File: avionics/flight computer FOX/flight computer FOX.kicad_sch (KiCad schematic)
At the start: 7 parts, among them U1 ESP32-S3-DevKitC

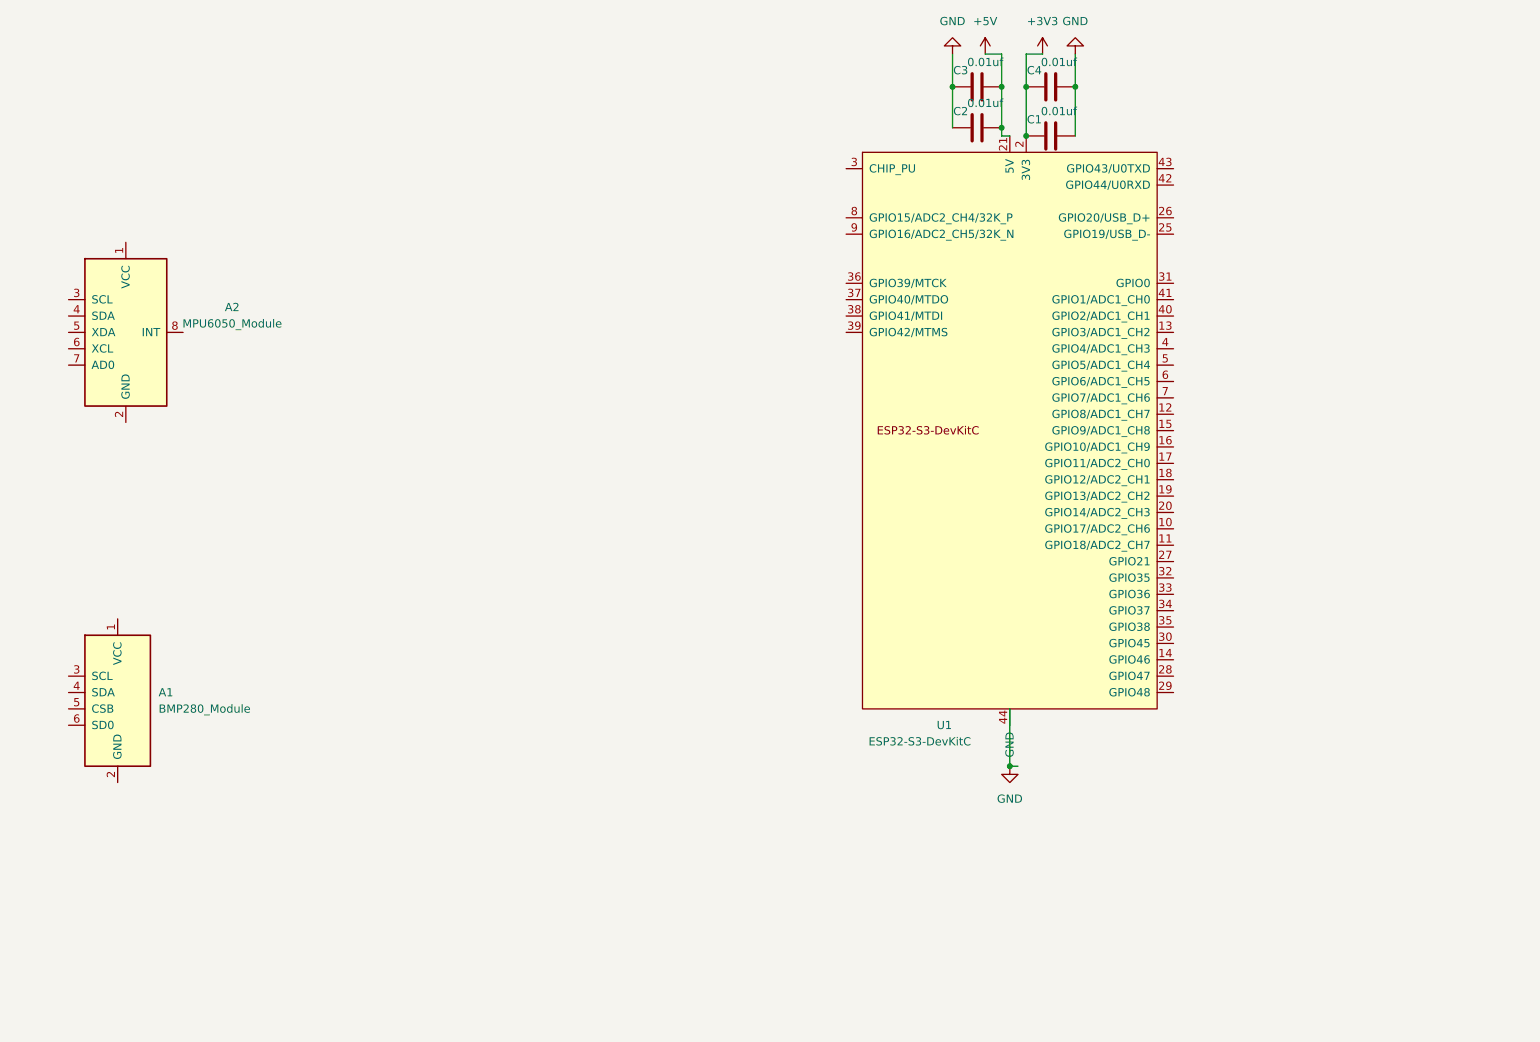
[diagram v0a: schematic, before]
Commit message: some stuff
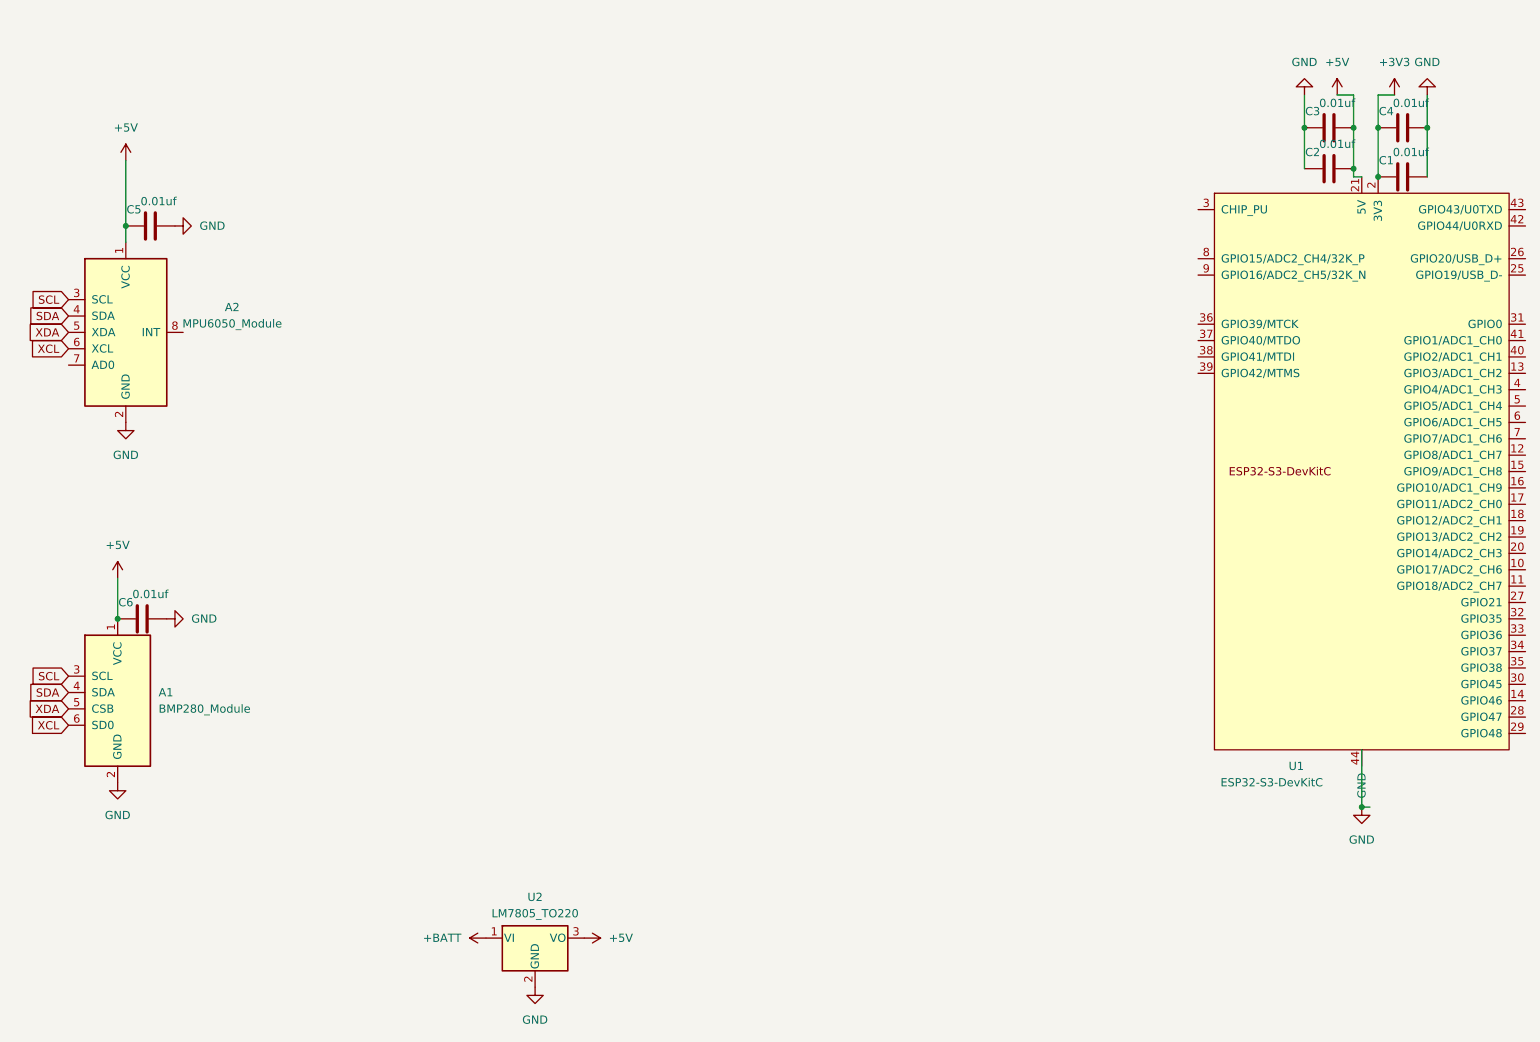
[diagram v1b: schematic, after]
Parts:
- added C5, C6: 0.01uf, symbol Device:C
- added U2: LM7805_TO220, Package_TO_SOT_THT:TO-220-3_Vertical, symbol Regulator_Linear:LM7805_TO220
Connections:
- net +5V: now also A1.1 (VCC), A2.1 (VCC), C5.1, C6.1, U2.3 (VO)
- net GND: now also A1.2 (GND), A2.2 (GND), C5.2, C6.2, U2.2 (GND)
- net SCL: now reaches A2.3 (SCL)
- net SCL: now also A1.3 (SCL)
- net SDA: now reaches A2.4 (SDA)
- net SDA: now also A1.4 (SDA)
- net XDA: now reaches A2.5 (XDA)
- net XDA: now also A1.5 (CSB)
- net XCL: now reaches A2.6 (XCL)
- net XCL: now also A1.6 (SD0)
- new net +BATT: U2.1 (VI)
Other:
- moved on the sheet: C1, C2, C3, C4, U1

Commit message: more flight computer work
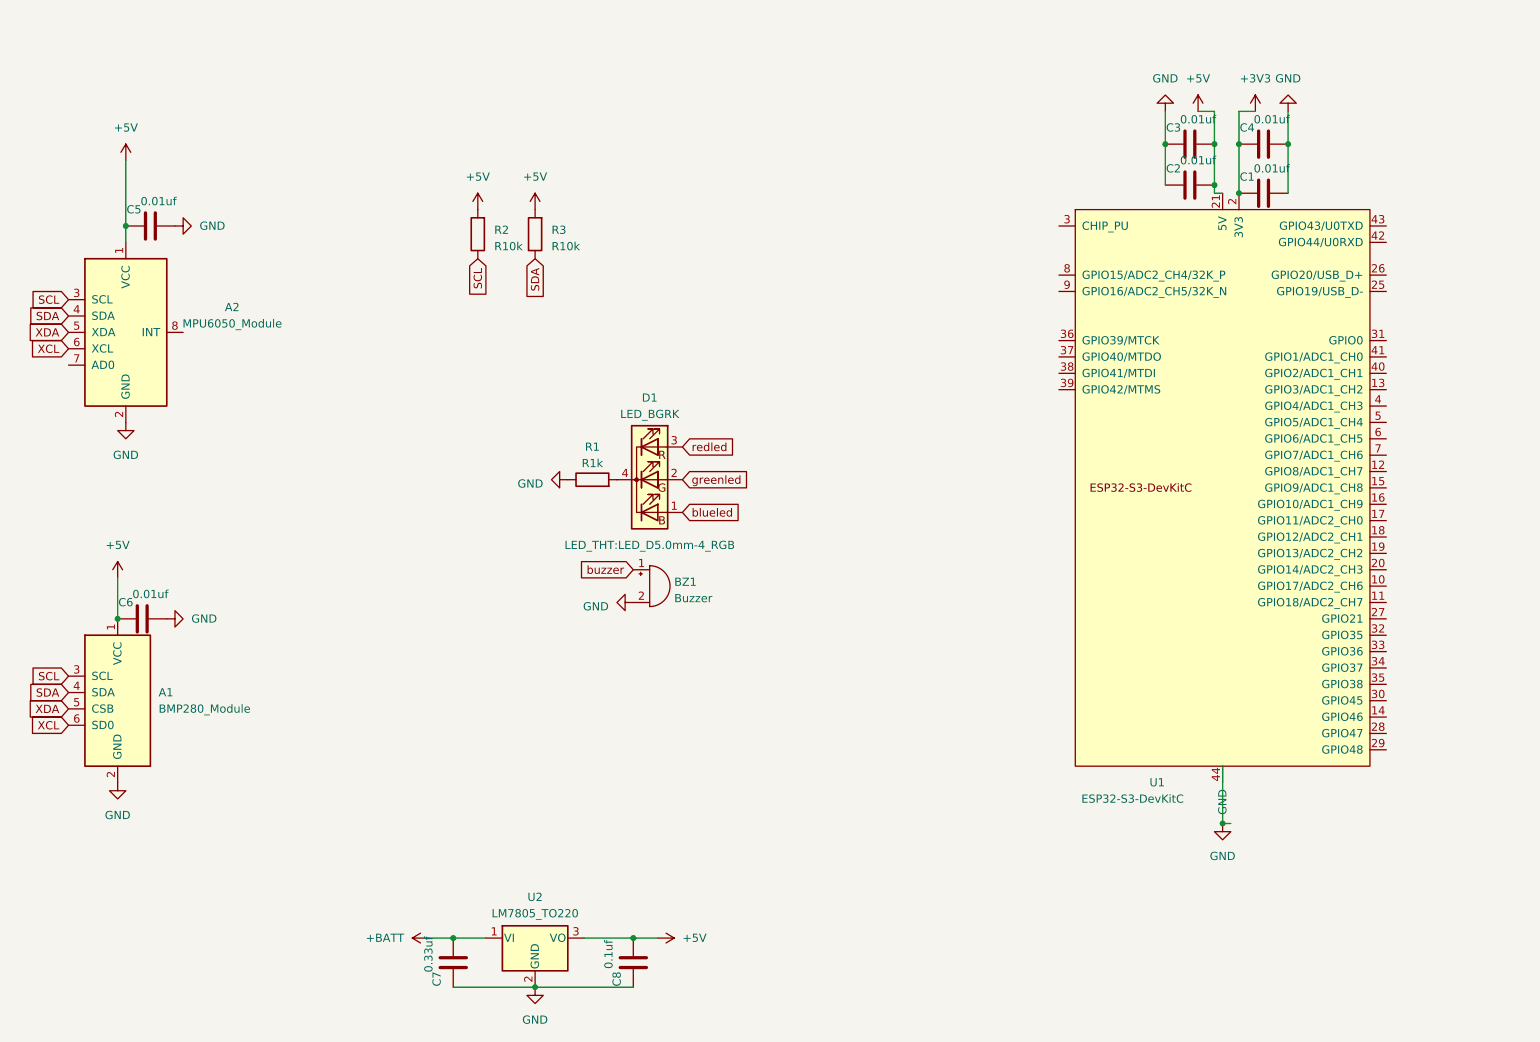
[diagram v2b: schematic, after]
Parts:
- added BZ1: Buzzer, Buzzer_Beeper:Buzzer_12x9.5RM7.6, symbol Device:Buzzer
- added C7: 0.33uf, Capacitor_SMD:C_0805_2012Metric_Pad1.18x1.45mm_HandSolder, symbol Device:C
- added C8: 0.1uf, Capacitor_SMD:C_0805_2012Metric_Pad1.18x1.45mm_HandSolder, symbol Device:C
- added D1: LED_BGRK, LED_THT:LED_D5.0mm-4_RGB, symbol Device:LED_BGRK
- added R1: R1k, symbol Device:R
- added R2, R3: R10k, symbol Device:R
- C1, C2, C3, C4, C5, C6: footprint (none) -> Capacitor_SMD:C_0805_2012Metric_Pad1.18x1.45mm_HandSolder
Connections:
- net +5V: now also C8.2, R2.2, R3.2
- net +BATT: now also C7.2
- net GND: now also BZ1.2 (+), C7.1, C8.1, R1.1
- net SCL: now also R2.1
- net SDA: now also R3.1
- new net: D1.4 (K), R1.2
- new net blueled: D1.1 (BA)
- new net buzzer: BZ1.1 (-)
- new net greenled: D1.2 (GA)
- new net redled: D1.3 (RA)
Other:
- moved on the sheet: C1, C2, C3, C4, U1

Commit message: more avionics work
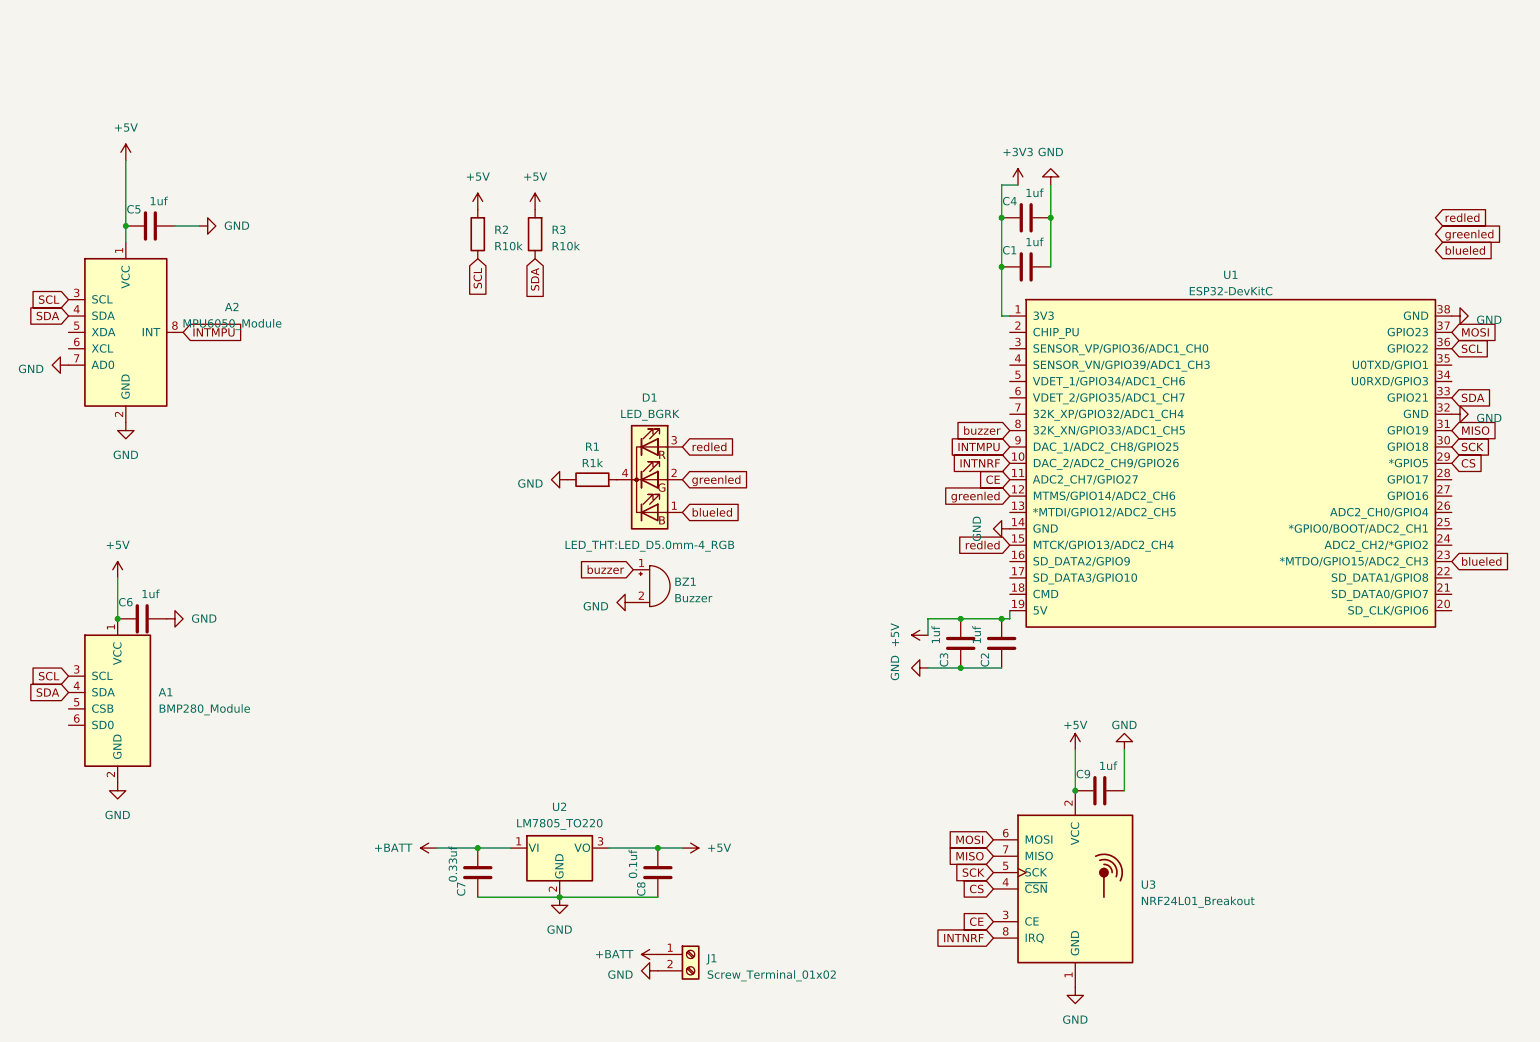
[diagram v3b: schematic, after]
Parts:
- removed U1: ESP32-S3-DevKitC, Espressif:ESP32-S3-DevKitC, symbol Espressif:ESP32-S3-DevKitC
- added C9: 1uf, Capacitor_SMD:C_0805_2012Metric_Pad1.18x1.45mm_HandSolder, symbol Device:C
- added J1: Screw_Terminal_01x02, TerminalBlock:TerminalBlock_bornier-2_P5.08mm, symbol Connector:Screw_Terminal_01x02
- added U1: ESP32-DevKitC, Espressif:ESP32-DevKitC, symbol Espressif:ESP32-DevKitC
- added U3: NRF24L01_Breakout, RF_Module:nRF24L01_Breakout, symbol RF:NRF24L01_Breakout
- C1, C2, C3, C4, C5, C6: value 0.01uf -> 1uf
- R1, R2, R3: footprint (none) -> Resistor_SMD:R_0805_2012Metric_Pad1.20x1.40mm_HandSolder
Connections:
- net +3V3: now also U1.1 (3V3)
- net +5V: now also C9.1, U1.19 (5V), U3.2 (VCC)
- net +BATT: now also J1.1 (Pin_1)
- net GND: now also A2.7 (AD0), C9.2, J1.2 (Pin_2), U1.14 (GND), U1.32 (GND), U1.38 (GND), U3.1 (GND)
- net SCL: now also U1.36 (GPIO22)
- net SDA: now also U1.33 (GPIO21)
- net blueled: now also U1.23 (*MTDO/GPIO15/ADC2_CH3)
- net buzzer: now also U1.8 (32K_XN/GPIO33/ADC1_CH5)
- net greenled: now also U1.12 (MTMS/GPIO14/ADC2_CH6)
- net redled: now also U1.15 (MTCK/GPIO13/ADC2_CH4)
- net INTMPU: now reaches A2.8 (INT)
- net INTMPU: now also U1.9 (DAC_1/ADC2_CH8/GPIO25)
- net XCL: no longer names the net of A2.6 (XCL)
- net XCL: no longer A1.6 (SD0)
- net XDA: no longer names the net of A2.5 (XDA)
- net XDA: no longer A1.5 (CSB)
- new net CE: U1.11 (ADC2_CH7/GPIO27), U3.3 (CE)
- new net CS: U1.29 (*GPIO5), U3.4 (~{CSN})
- new net INTNRF: U1.10 (DAC_2/ADC2_CH9/GPIO26), U3.8 (IRQ)
- new net MISO: U1.31 (GPIO19), U3.7 (MISO)
- new net MOSI: U1.37 (GPIO23), U3.6 (MOSI)
- new net SCK: U1.30 (GPIO18), U3.5 (SCK)
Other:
- moved on the sheet: C1, C2, C3, C4, C7, C8, U2
